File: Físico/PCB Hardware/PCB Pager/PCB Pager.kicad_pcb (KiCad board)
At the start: 2 copper layers, 66.5 x 82.8 mm, 13 parts, among them J1 Conn_01x06_Male, J2 Conn_01x06_Male, J3 Conn_01x04_Female, J6 Screw_Terminal_01x02, SW1 SW_Push, SW2 SW_Push, SW3 SW_Push, U1 L7805, U2 ESP32-DEVKIT-V1

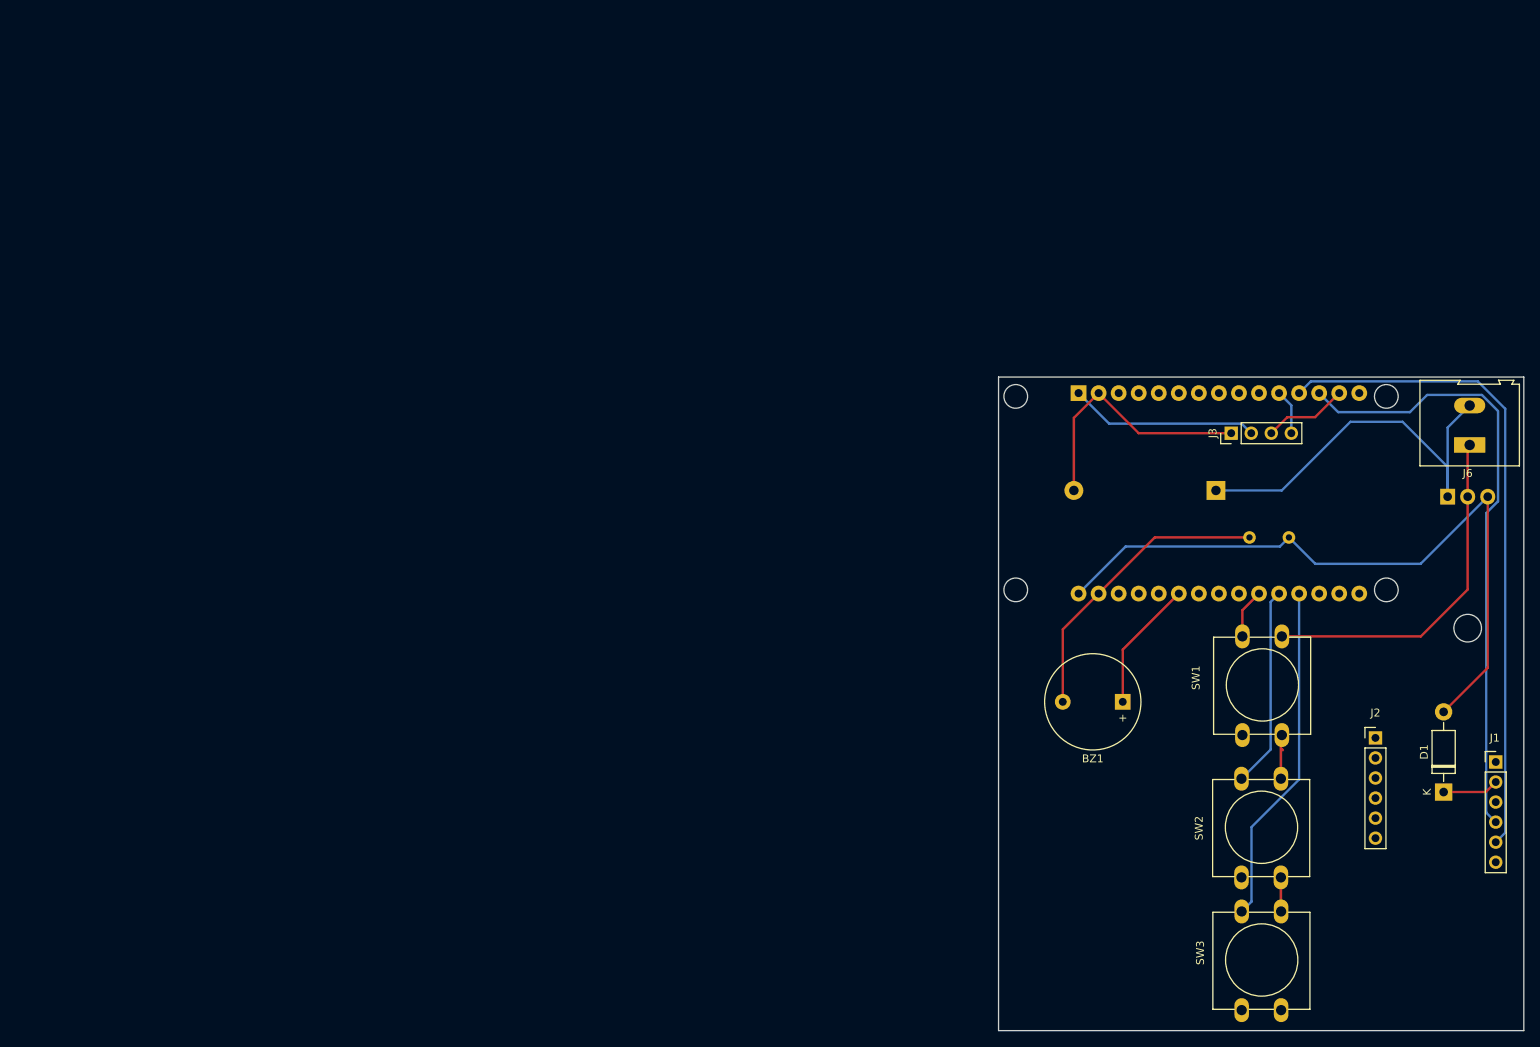
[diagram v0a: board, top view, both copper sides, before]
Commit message: Atualização Parada e Placa Prontas
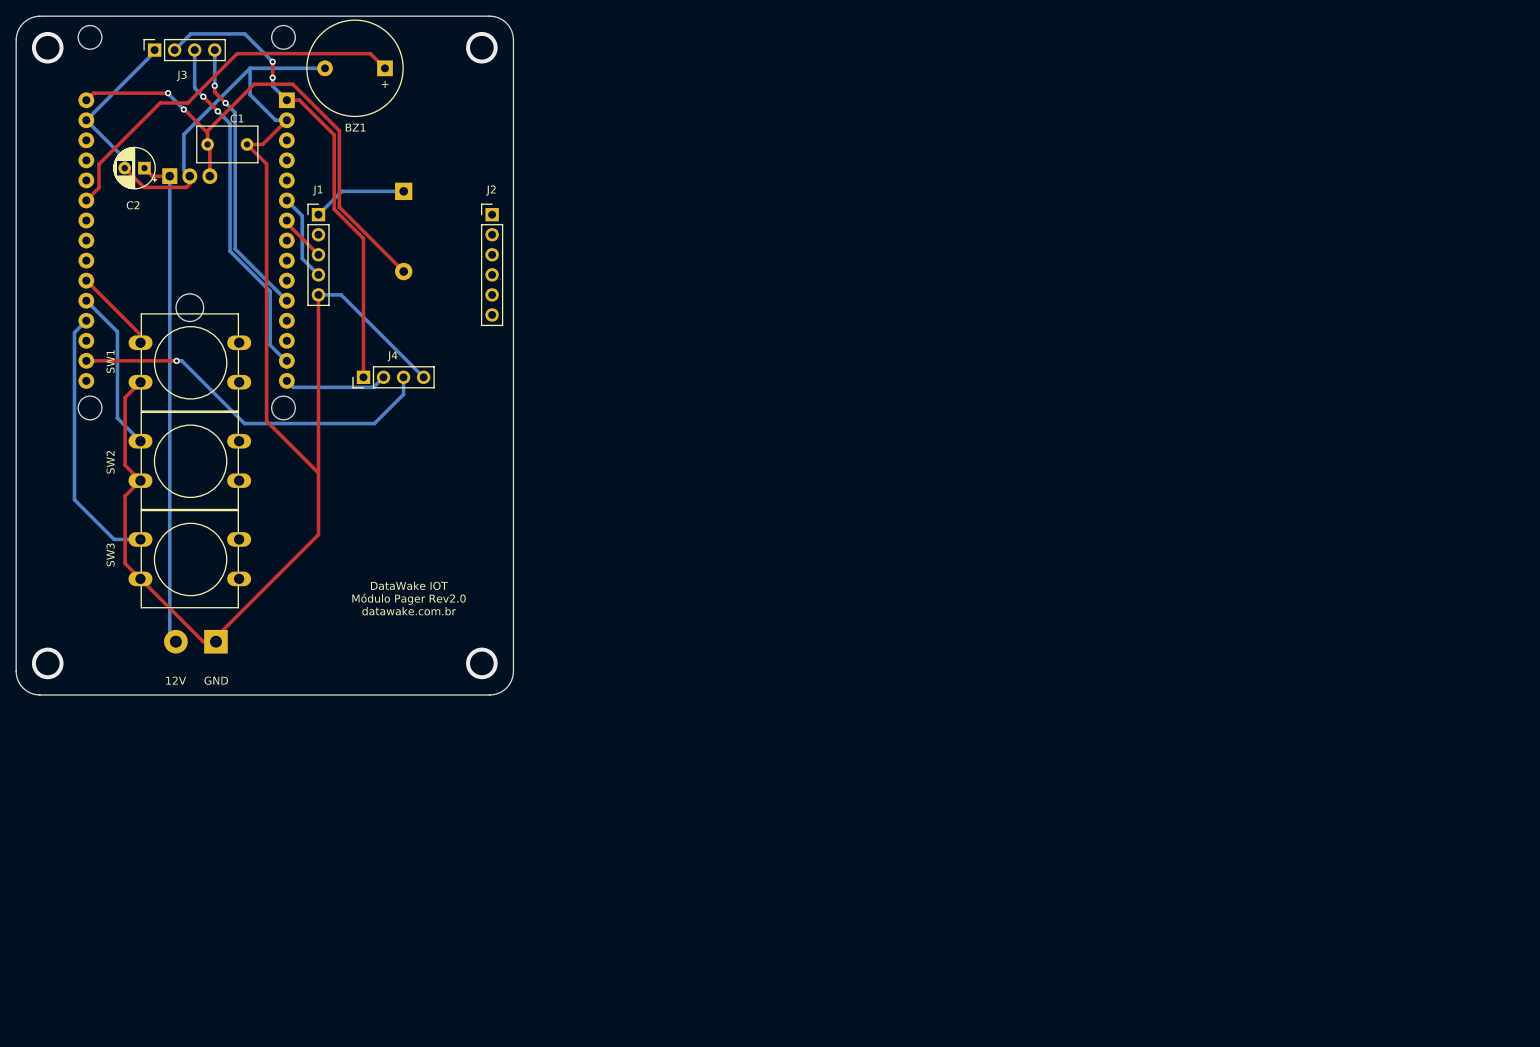
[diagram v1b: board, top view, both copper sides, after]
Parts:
- added J4: Conn_01x04_Male, Connector_PinHeader_2.54mm:PinHeader_1x04_P2.54mm_Vertical, F.Cu at (44.0, 45.8)
- C1: moved to F.Cu
- C2: footprint Capacitor_THT:CP_Axial_L11.0mm_D6.0mm_P18.00mm_Horizontal -> Capacitor_THT:CP_Radial_D5.0mm_P2.50mm; moved to F.Cu
- D1: moved to B.Cu
- J1: value Conn_01x06_Male -> Conn_01x05_Male; footprint Connector_PinHeader_2.54mm:PinHeader_1x06_P2.54mm_Vertical -> Connector_PinHeader_2.54mm:PinHeader_1x05_P2.54mm_Vertical
- J3: footprint Connector_PinHeader_2.54mm:PinHeader_1x04_P2.54mm_Vertical -> Connector_PinSocket_2.54mm:PinSocket_1x04_P2.54mm_Vertical
- J6: footprint TerminalBlock:TerminalBlock_Altech_AK300-2_P5.00mm -> TerminalBlock:TerminalBlock_bornier-2_P5.08mm; moved to B.Cu
- moved U1 166.9 mm to (19.5, 20.3)
- moved J1 164.5 mm to (38.3, 25.1)
- moved J6 160.8 mm to (25.3, 79.2), turned to 180 degrees
- moved D1 152.1 mm to (49.1, 22.2), turned to -90 degrees
- moved SW3 151.7 mm to (15.7, 66.3), turned to 0 degrees
- moved SW2 150.0 mm to (15.7, 53.8), turned to 0 degrees
- moved SW1 148.2 mm to (15.8, 41.4), turned to 0 degrees
- moved C1 145.8 mm to (24.2, 16.2), turned to 0 degrees
- moved J3 144.8 mm to (17.5, 4.29)
- moved C2 141.8 mm to (16.2, 19.2)
- moved U2 133.0 mm to (21.6, 26.2), turned to 180 degrees
- moved J2 130.1 mm to (60.3, 25.1)
- moved BZ1 123.2 mm to (46.7, 6.60)
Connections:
- D1 pad 1: Net-(J1-Pad2) -> Net-(D1-Pad1)
- J1 pad 1: unconnected-(J1-Pad1) -> Net-(D1-Pad1)
- J1 pad 2: Net-(J1-Pad2) -> unconnected-(J1-Pad2)
- J1 pad 3: unconnected-(J1-Pad3) -> RXD
- J1 pad 4: RXD -> TXD
- J1 pad 5: TXD -> Earth
- U2 pad 12: TXD -> unconnected-(U2-Pad12)
- U2 pad 13: RXD -> unconnected-(U2-Pad13)
- U2 pad 15: unconnected-(U2-Pad15) -> RX2
- U2 pad 17: unconnected-(U2-Pad17) -> TX2
- U2 pad 6: unconnected-(U2-Pad6) -> TXD
- U2 pad 7: unconnected-(U2-Pad7) -> RXD
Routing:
- net Earth: track 124.7 -> 226.5 mm
- net RXD: track 78.6 -> 6.00 mm
- net TXD: track 83.6 -> 11.1 mm
- net TX2: track 0.00 -> 47.2 mm, vias 0 -> 1
- net 3.3V: track 24.0 -> 60.4 mm, vias 0 -> 2
- net Net-(J3-Pad3): track 10.7 -> 44.3 mm, vias 0 -> 2
- net GPIO27: track 16.7 -> 48.1 mm
- net Net-(J3-Pad4): track 5.72 -> 35.5 mm, vias 0 -> 2
- net 5V: track 89.3 -> 66.4 mm, vias 0 -> 2
- net RX2: track 0.00 -> 13.1 mm
- net Net-(D1-Pad1): track 0.00 -> 12.0 mm
- net 12V: track 51.8 -> 62.8 mm
- net GPIO34: track 43.3 -> 33.7 mm
- net Net-(J1-Pad2): track 7.13 -> 0.00 mm
- net GPIO35: track 25.4 -> 20.6 mm
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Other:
- board size 66.5 x 82.8 mm -> 63 x 86 mm
- board text added: "12V"
- board text added: "DataWake IOT Módulo Pager Rev2.0 datawake.com.br"
- board text added: "GND"
